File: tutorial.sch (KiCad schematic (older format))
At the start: 4 parts

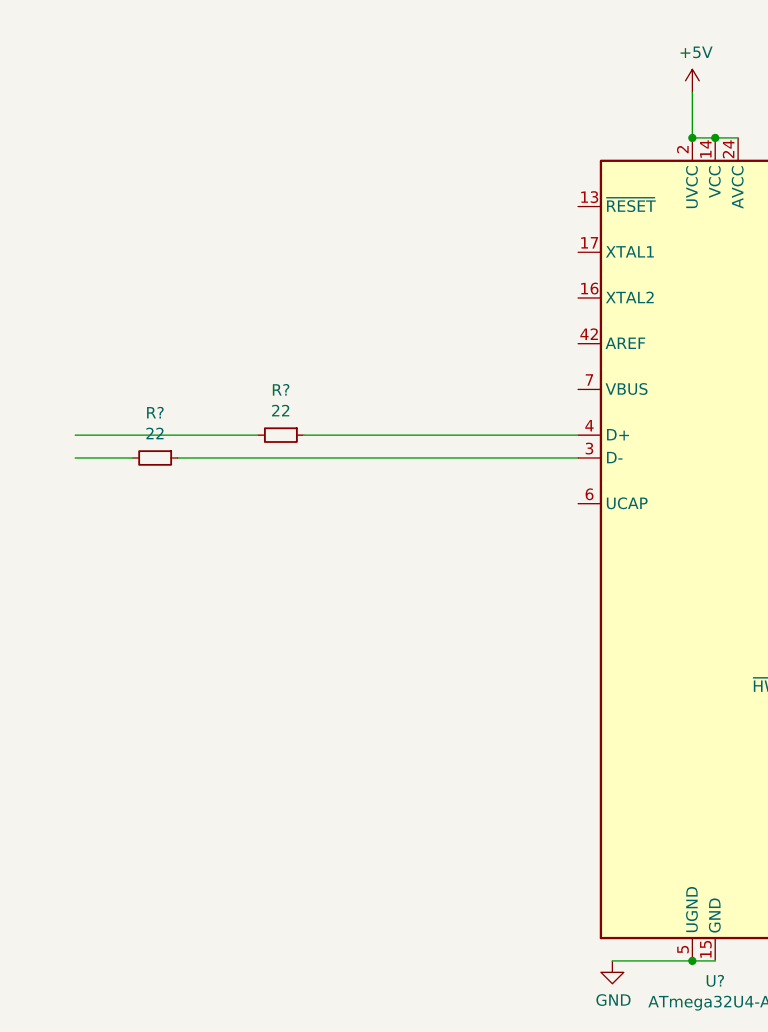
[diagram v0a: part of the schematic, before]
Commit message: Finished MCU
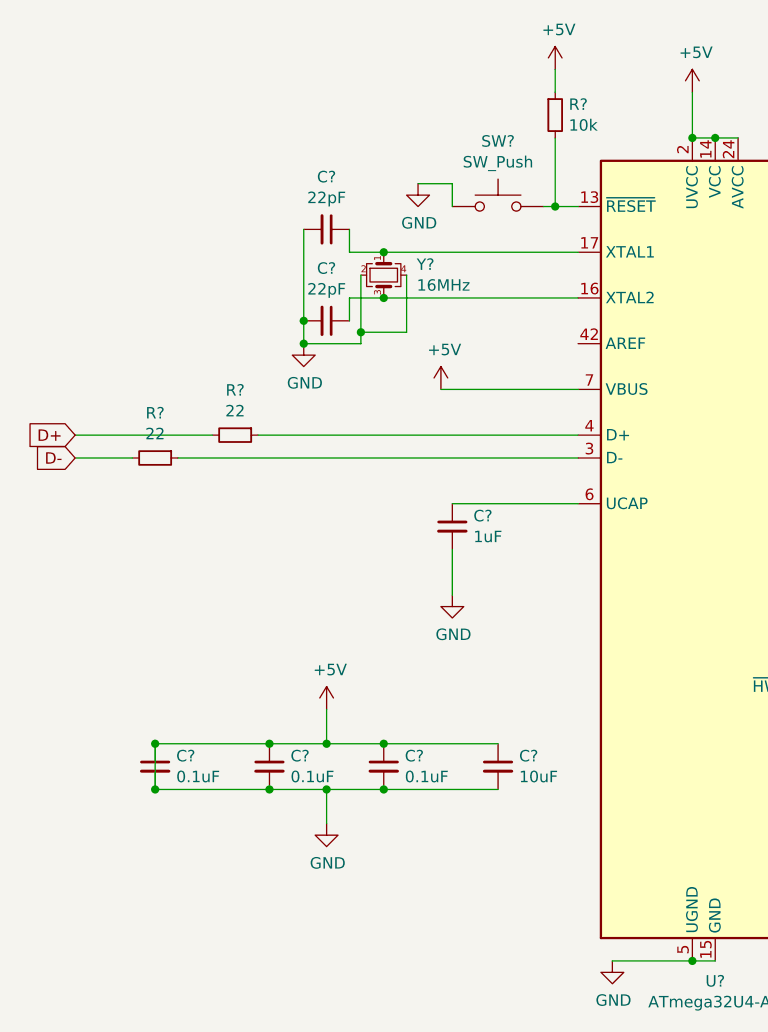
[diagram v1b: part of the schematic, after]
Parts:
- added C?: 1uF, symbol Device:C_Small
- added C?: 10uF, symbol Device:C_Small
- added C? (x3): 0.1uF, symbol Device:C_Small
- added C? (x2): 22pF, symbol Device:C_Small
- added R?: 10k, symbol Device:R_Small
- added SW?: SW_Push, symbol Switch:SW_Push
- added Y?: 16MHz, symbol Device:Crystal_GND24_Small
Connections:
- net labels added: D+, D-
- wire segments 11 -> 44
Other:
- moved on the sheet: R?

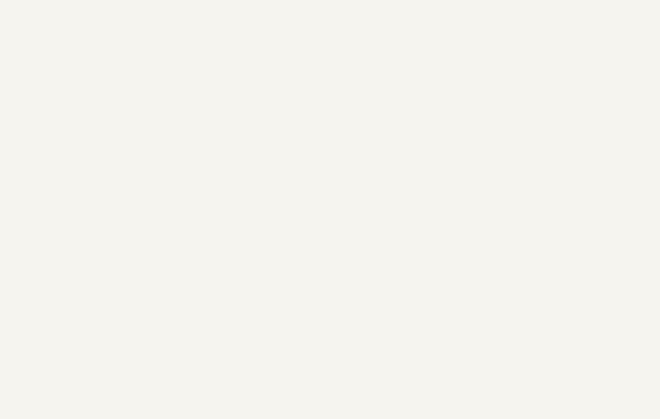
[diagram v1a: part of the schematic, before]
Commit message: USB
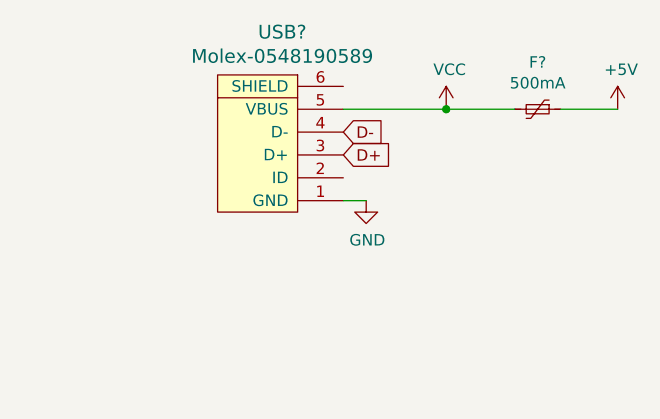
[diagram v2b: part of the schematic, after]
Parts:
- added F?: 500mA, symbol Device:Polyfuse_Small
- added USB?: Molex-0548190589, symbol random-keyboard-parts:Molex-0548190589
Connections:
- net +5V: now also F?.1, USB?.1 (GND)
- net D+: now also USB?.3 (D+)
- net D-: now also USB?.4 (D-)
- new net VCC: F?.2, USB?.5 (VBUS)
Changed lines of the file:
@@
 	0    1    1    0
 $EndComp
+$Comp
+L random-keyboard-parts:Molex-0548190589 USB?
+U 1 1 5F3A7983
+P 8350 1850
+F 0 "USB?" V 8887 1817 60  0000 C CNN
+F 1 "Molex-0548190589" V 8781 1817 60  0000 C CNN
+F 2 "" H 8350 1850 60  0001 C CNN
+F 3 "" H 8350 1850 60  0001 C CNN
+	1    8350 1850
+	0    -1   -1   0
+$EndComp
+$Comp
+L power:VCC #PWR?
+U 1 1 5F3A8DEB
+P 9100 1650
+F 0 "#PWR?" H 9100 1500 50  0001 C CNN
+F 1 "VCC" H 9115 1823 50  0000 C CNN
+F 2 "" H 9100 1650 50  0001 C CNN
+F 3 "" H 9100 1650 50  0001 C CNN
+	1    9100 1650
+	1    0    0    -1
+$EndComp
+$Comp
+L Device:Polyfuse_Small F?
+U 1 1 5F3AA1DA
+P 9500 1650
+F 0 "F?" V 9295 1650 50  0000 C CNN
+F 1 "500mA" V 9386 1650 50  0000 C CNN
+F 2 "" H 9550 1450 50  0001 L CNN
+F 3 "~" H 9500 1650 50  0001 C CNN
+	1    9500 1650
+	0    1    1    0
+$EndComp
+$Comp
+L power:+5V #PWR?
+U 1 1 5F3AADB2
+P 9850 1650
+F 0 "#PWR?" H 9850 1500 50  0001 C CNN
+F 1 "+5V" H 9865 1823 50  0000 C CNN
+F 2 "" H 9850 1650 50  0001 C CNN
+F 3 "" H 9850 1650 50  0001 C CNN
+	1    9850 1650
+	1    0    0    -1
+$EndComp
+Wire Wire Line
+	8650 1650 9100 1650
+Connection ~ 9100 1650
+Wire Wire Line
+	9100 1650 9400 1650
+Wire Wire Line
+	9600 1650 9850 1650
+Text GLabel 8650 1750 2    50   Input ~ 0
+D-
+Text GLabel 8650 1850 2    50   Input ~ 0
+D+
+$Comp
+L power:GND #PWR?
+U 1 1 5F3AE84A
+P 8750 2050
+F 0 "#PWR?" H 8750 1800 50  0001 C CNN
+F 1 "GND" H 8755 1877 50  0000 C CNN
+F 2 "" H 8750 2050 50  0001 C CNN
+F 3 "" H 8750 2050 50  0001 C CNN
+	1    8750 2050
+	1    0    0    -1
+$EndComp
+Wire Wire Line
+	8650 2050 8750 2050
 $EndSCHEMATC

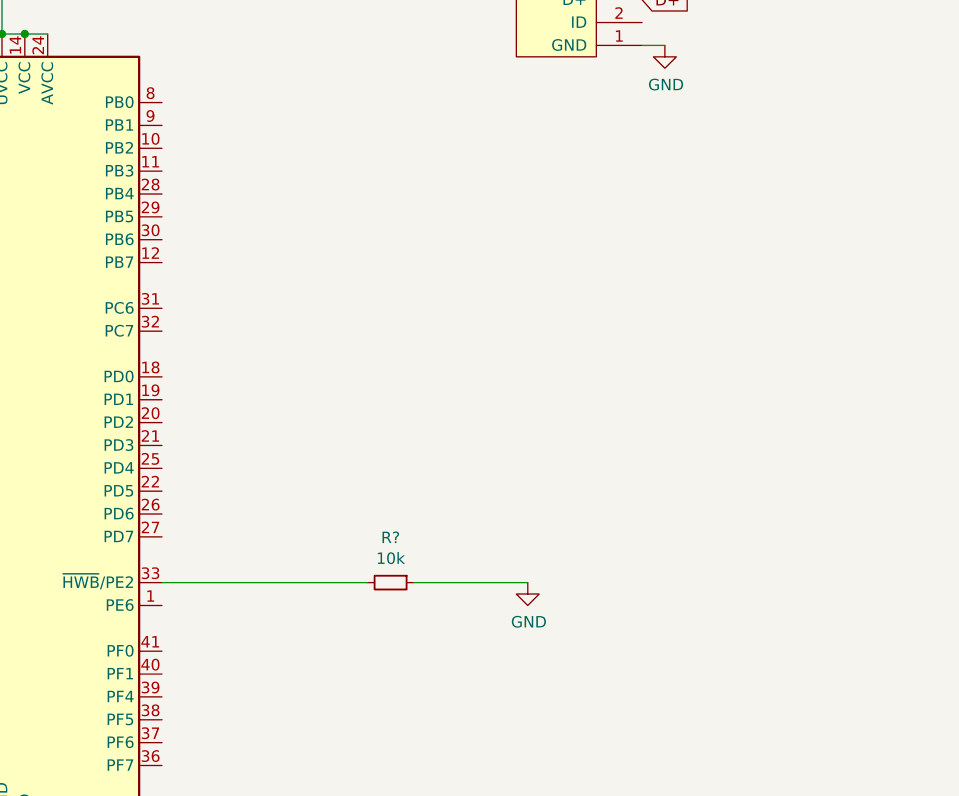
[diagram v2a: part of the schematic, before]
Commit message: Matrix
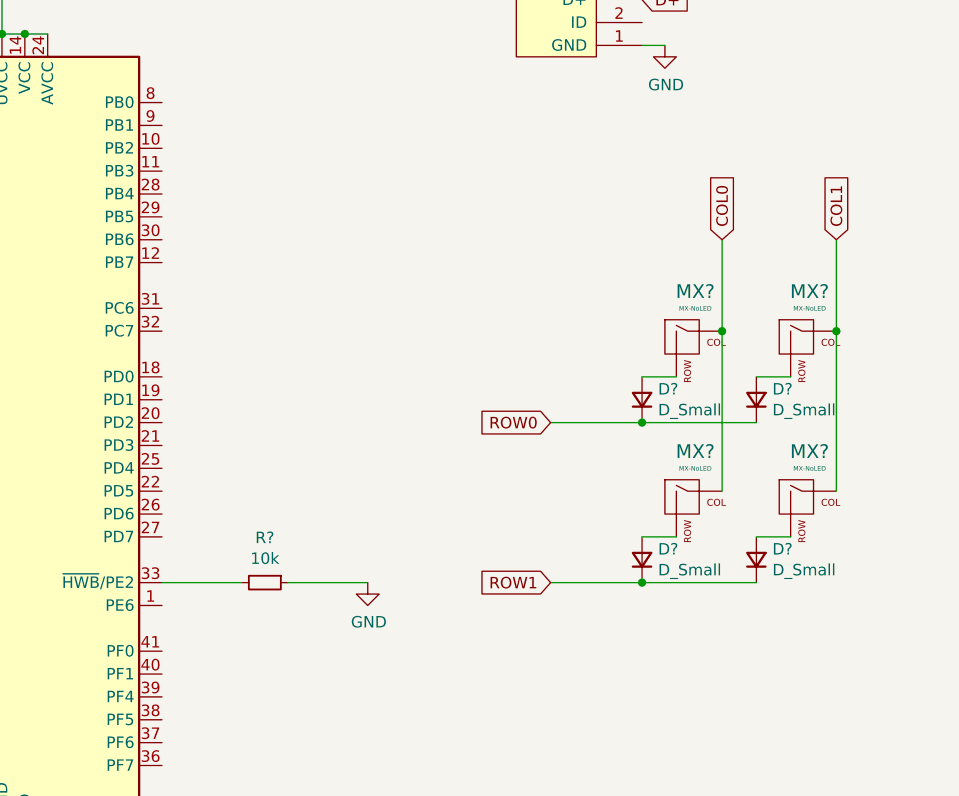
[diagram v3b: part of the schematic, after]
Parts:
- added D? (x4): D_Small, symbol Device:D_Small
- added MX? (x4): MX-NoLED, symbol MX_Alps_Hybrid:MX-NoLED
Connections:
- new net: D?.2 (A), MX?.2 (ROW) (x4)
- new net COL0: MX?.1 (COL), MX?.1 (COL)
- new net COL1: MX?.1 (COL), MX?.1 (COL)
- new net ROW0: D?.1 (K), D?.1 (K)
- new net ROW1: D?.1 (K), D?.1 (K)
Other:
- moved on the sheet: R?
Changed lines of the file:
@@
 L power:GND #PWR?
 U 1 1 5F377EA3
-P 8150 4400
-F 0 "#PWR?" H 8150 4150 50  0001 C CNN
-F 1 "GND" H 8155 4227 50  0000 C CNN
-F 2 "" H 8150 4400 50  0001 C CNN
-F 3 "" H 8150 4400 50  0001 C CNN
-	1    8150 4400
-	1    0    0    -1
-$EndComp
-Wire Wire Line
-	7650 4400 8150 4400
-Wire Wire Line
-	6550 4400 7450 4400
+P 7450 4400
+F 0 "#PWR?" H 7450 4150 50  0001 C CNN
+F 1 "GND" H 7455 4227 50  0000 C CNN
+F 2 "" H 7450 4400 50  0001 C CNN
+F 3 "" H 7450 4400 50  0001 C CNN
+	1    7450 4400
+	1    0    0    -1
+$EndComp
 $Comp
 L Device:R_Small R?
 U 1 1 5F3767D8
-P 7550 4400
-F 0 "R?" V 7354 4400 50  0000 C CNN
-F 1 "10k" V 7445 4400 50  0000 C CNN
-F 2 "" H 7550 4400 50  0001 C CNN
-F 3 "~" H 7550 4400 50  0001 C CNN
-	1    7550 4400
+P 7000 4400
+F 0 "R?" V 6804 4400 50  0000 C CNN
+F 1 "10k" V 6895 4400 50  0000 C CNN
+F 2 "" H 7000 4400 50  0001 C CNN
+F 3 "~" H 7000 4400 50  0001 C CNN
+	1    7000 4400
 	0    1    1    0
 $EndComp
@@
 Wire Wire Line
 	8650 2050 8750 2050
+Wire Wire Line
+	6550 4400 6900 4400
+Wire Wire Line
+	7100 4400 7450 4400
+$Comp
+L MX_Alps_Hybrid:MX-NoLED MX?
+U 1 1 5F3B1ED5
+P 8850 3350
+F 0 "MX?" H 8883 3573 60  0000 C CNN
+F 1 "MX-NoLED" H 8883 3499 20  0000 C CNN
+F 2 "" H 8225 3325 60  0001 C CNN
+F 3 "" H 8225 3325 60  0001 C CNN
+	1    8850 3350
+	1    0    0    -1
+$EndComp
+$Comp
+L Device:D_Small D?
+U 1 1 5F3B2F2B
+P 8650 3600
+F 0 "D?" V 8696 3530 50  0000 R CNN
+F 1 "D_Small" V 8605 3530 50  0000 R CNN
+F 2 "" V 8650 3600 50  0001 C CNN
+F 3 "~" V 8650 3600 50  0001 C CNN
+	1    8650 3600
+	0    -1   -1   0
+$EndComp
+Wire Wire Line
+	8800 3500 8650 3500
+$Comp
+L MX_Alps_Hybrid:MX-NoLED MX?
+U 1 1 5F3B561A
+P 9350 3350
+F 0 "MX?" H 9383 3573 60  0000 C CNN
+F 1 "MX-NoLED" H 9383 3499 20  0000 C CNN
+F 2 "" H 8725 3325 60  0001 C CNN
+F 3 "" H 8725 3325 60  0001 C CNN
+	1    9350 3350
+	1    0    0    -1
+$EndComp
+$Comp
+L Device:D_Small D?
+U 1 1 5F3B5620
+P 9150 3600
+F 0 "D?" V 9196 3530 50  0000 R CNN
+F 1 "D_Small" V 9105 3530 50  0000 R CNN
+F 2 "" V 9150 3600 50  0001 C CNN
+F 3 "~" V 9150 3600 50  0001 C CNN
+	1    9150 3600
+	0    -1   -1   0
+$EndComp
+Wire Wire Line
+	9300 3500 9150 3500
+$Comp
+L MX_Alps_Hybrid:MX-NoLED MX?
+U 1 1 5F3B8106
+P 9350 4050
+F 0 "MX?" H 9383 4273 60  0000 C CNN
+F 1 "MX-NoLED" H 9383 4199 20  0000 C CNN
+F 2 "" H 8725 4025 60  0001 C CNN
+F 3 "" H 8725 4025 60  0001 C CNN
+	1    9350 4050
+	1    0    0    -1
+$EndComp
+$Comp
+L Device:D_Small D?
+U 1 1 5F3B810C
+P 9150 4300
+F 0 "D?" V 9196 4230 50  0000 R CNN
+F 1 "D_Small" V 9105 4230 50  0000 R CNN
+F 2 "" V 9150 4300 50  0001 C CNN
+F 3 "~" V 9150 4300 50  0001 C CNN
+	1    9150 4300
+	0    -1   -1   0
+$EndComp
+Wire Wire Line
+	9300 4200 9150 4200
+$Comp
+L MX_Alps_Hybrid:MX-NoLED MX?
+U 1 1 5F3B9287
+P 8850 4050
+F 0 "MX?" H 8883 4273 60  0000 C CNN
+F 1 "MX-NoLED" H 8883 4199 20  0000 C CNN
+F 2 "" H 8225 4025 60  0001 C CNN
+F 3 "" H 8225 4025 60  0001 C CNN
+	1    8850 4050
+	1    0    0    -1
+$EndComp
+$Comp
+L Device:D_Small D?
+U 1 1 5F3B928D
+P 8650 4300
+F 0 "D?" V 8696 4230 50  0000 R CNN
+F 1 "D_Small" V 8605 4230 50  0000 R CNN
+F 2 "" V 8650 4300 50  0001 C CNN
+F 3 "~" V 8650 4300 50  0001 C CNN
+	1    8650 4300
+	0    -1   -1   0
+$EndComp
+Wire Wire Line
+	8800 4200 8650 4200
+Wire Wire Line
+	9500 4000 9500 3300
+Connection ~ 9500 3300
+Wire Wire Line
+	9500 3300 9500 2900
+Wire Wire Line
+	9000 4000 9000 3300
+Connection ~ 9000 3300
+Wire Wire Line
+	9000 3300 9000 2900
+Wire Wire Line
+	9150 3700 8650 3700
+Connection ~ 8650 3700
+Wire Wire Line
+	8650 3700 8250 3700
+Wire Wire Line
+	9150 4400 8650 4400
+Connection ~ 8650 4400
+Wire Wire Line
+	8650 4400 8250 4400
+Text GLabel 9000 2900 1    50   Input ~ 0
+COL0
+Text GLabel 9500 2900 1    50   Input ~ 0
+COL1
+Text GLabel 8250 3700 0    50   Input ~ 0
+ROW0
+Text GLabel 8250 4400 0    50   Input ~ 0
+ROW1
 $EndSCHEMATC
